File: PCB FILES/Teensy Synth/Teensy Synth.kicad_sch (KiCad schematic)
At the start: 132 parts, among them J1 Conn_01x05, J2 Conn_01x11_Socket, J2 USB_BOOT, J3 RST, J4 Conn_01x04, SW1 SW_Push, SW10 SW_Push, SW11 SW_Push, SW12 SW_Push, SW13 SW_Push, SW14 SW_Push, SW15 SW_Push, SW16 SW_Push, SW17 SW_Push, SW18 SW_Push, SW19 SW_Push, SW2 SW_Push, SW20 SW_Push, SW21 SW_Push, SW22 SW_Push, SW23 SW_Push, SW24 SW_Push, SW25 SW_Push, SW26 SW_Push, SW27 SW_Push, SW28 SW_Push, SW29 SW_Push, SW3 SW_Push, SW30 SW_Push, SW31 SW_Push, SW32 SW_Push, SW33 SW_Push, SW34 SW_Push, SW35 SW_Push, SW36 SW_Push, SW37 SW_Push, SW38 SW_Push, SW39 SW_Push, SW4 SW_Push, SW40 SW_Push, SW41 SW_Push, SW42 SW_Push, SW43 SW_Push, SW44 SW_Push, SW45 SW_Push, SW46 SW_Push, SW47 SW_Push, SW48 RotaryEncoder, SW49 RotaryEncoder, SW5 SW_Push, SW50 RotaryEncoder, SW51 RotaryEncoder, SW52 RotaryEncoder, SW6 SW_Push, SW7 SW_Push, SW8 SW_Push, SW9 SW_Push, U1 RP2040, U1 Teensy4.1, U2 NCP1117-3.3_SOT223, U2 TPS61090, U3 W25Q128JVS, U6 MCP73871, Y1 Crystal_Small

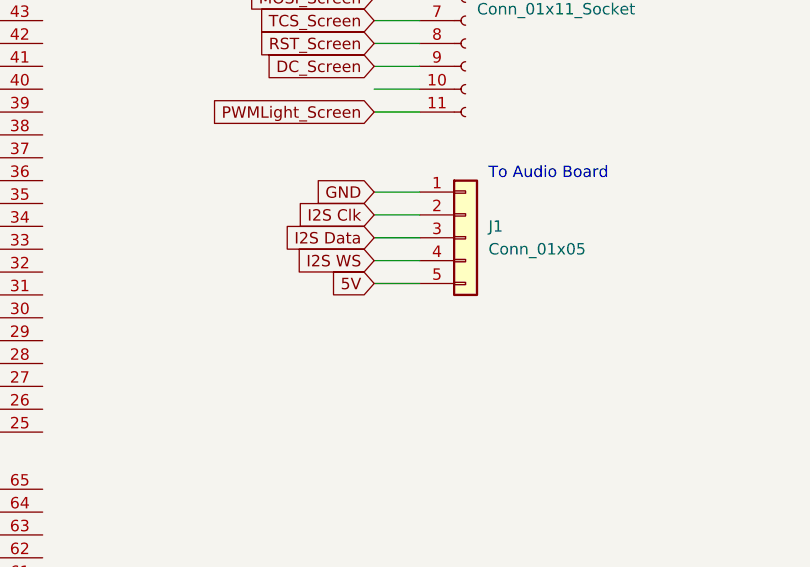
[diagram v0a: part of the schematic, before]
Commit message: VAL PLS CONNECT AND COMMIT
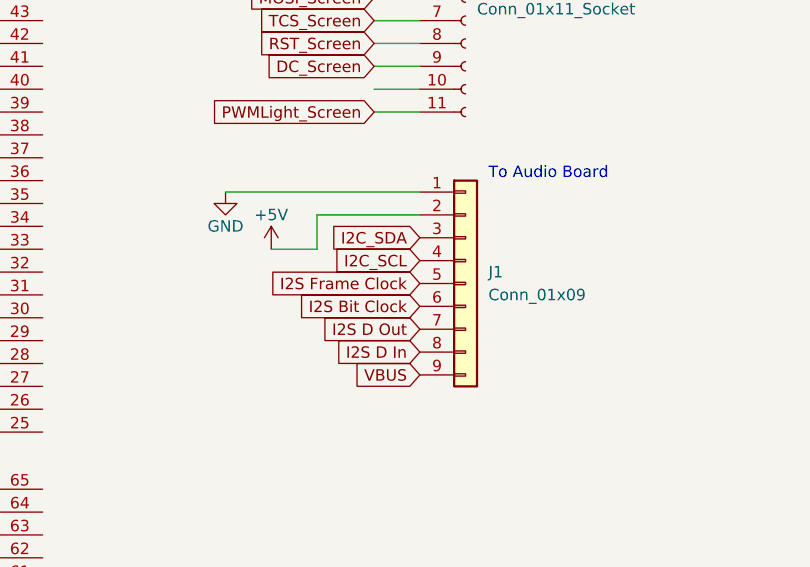
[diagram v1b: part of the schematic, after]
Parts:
- removed J1: Conn_01x05, symbol Connector_Generic:Conn_01x05
- added J1: Conn_01x09, Connector_JST:JST_SH_SM09B-SRSS-TB_1x09-1MP_P1.00mm_Horizontal, symbol Connector_Generic:Conn_01x09
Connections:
- net +5V: now also J1.2 (Pin_2)
- net GND: now also J1.1 (Pin_1)
- net VBUS: now also J1.9 (Pin_9)
- new net I2C_SCL: J1.4 (Pin_4)
- new net I2C_SDA: J1.3 (Pin_3)
- new net I2S Bit Clock: J1.6 (Pin_6)
- new net I2S D In: J1.8 (Pin_8)
- new net I2S D Out: J1.7 (Pin_7)
- new net I2S Frame Clock: J1.5 (Pin_5)
